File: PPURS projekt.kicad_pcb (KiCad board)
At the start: 2 copper layers, 80.5 x 53.5 mm, 26 parts, among them J3 Barrel_Jack, SW1 SW_Push_Dual, Y1 8Mhz

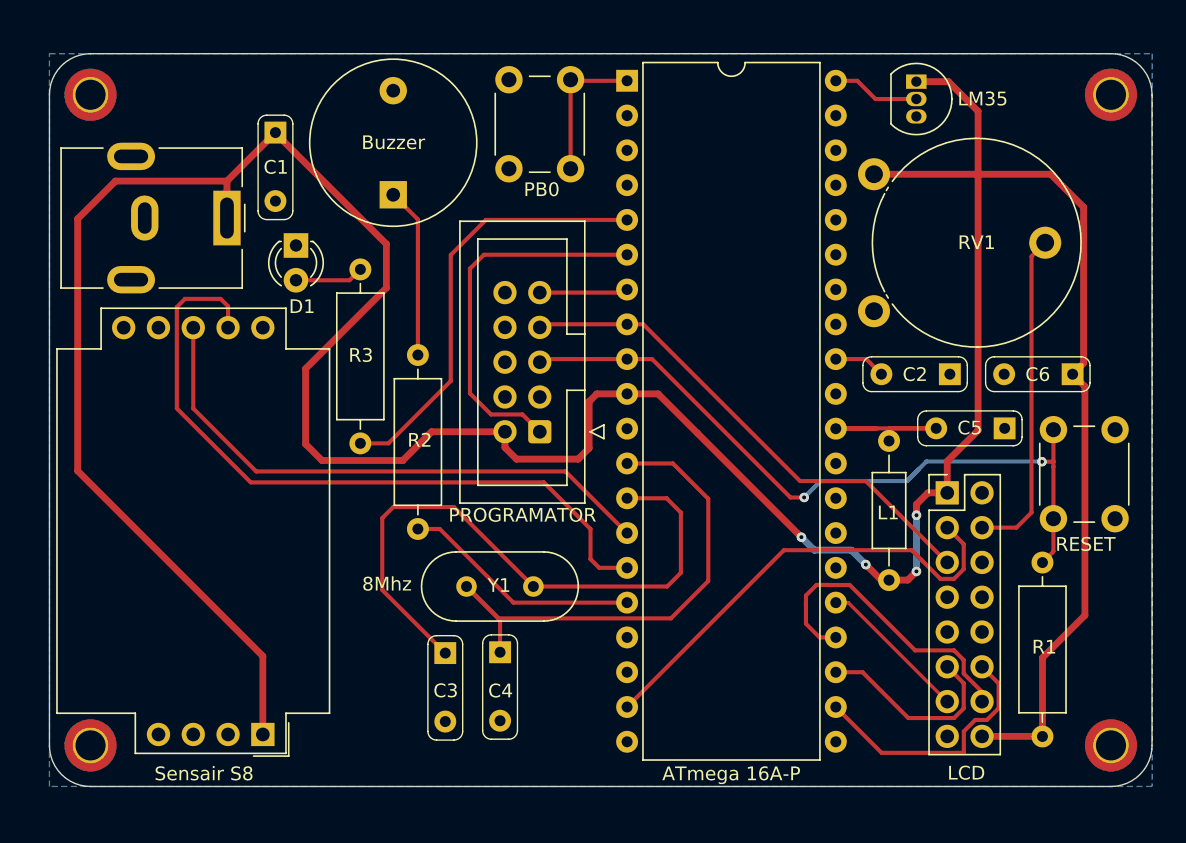
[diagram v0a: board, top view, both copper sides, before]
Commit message: Add files via upload
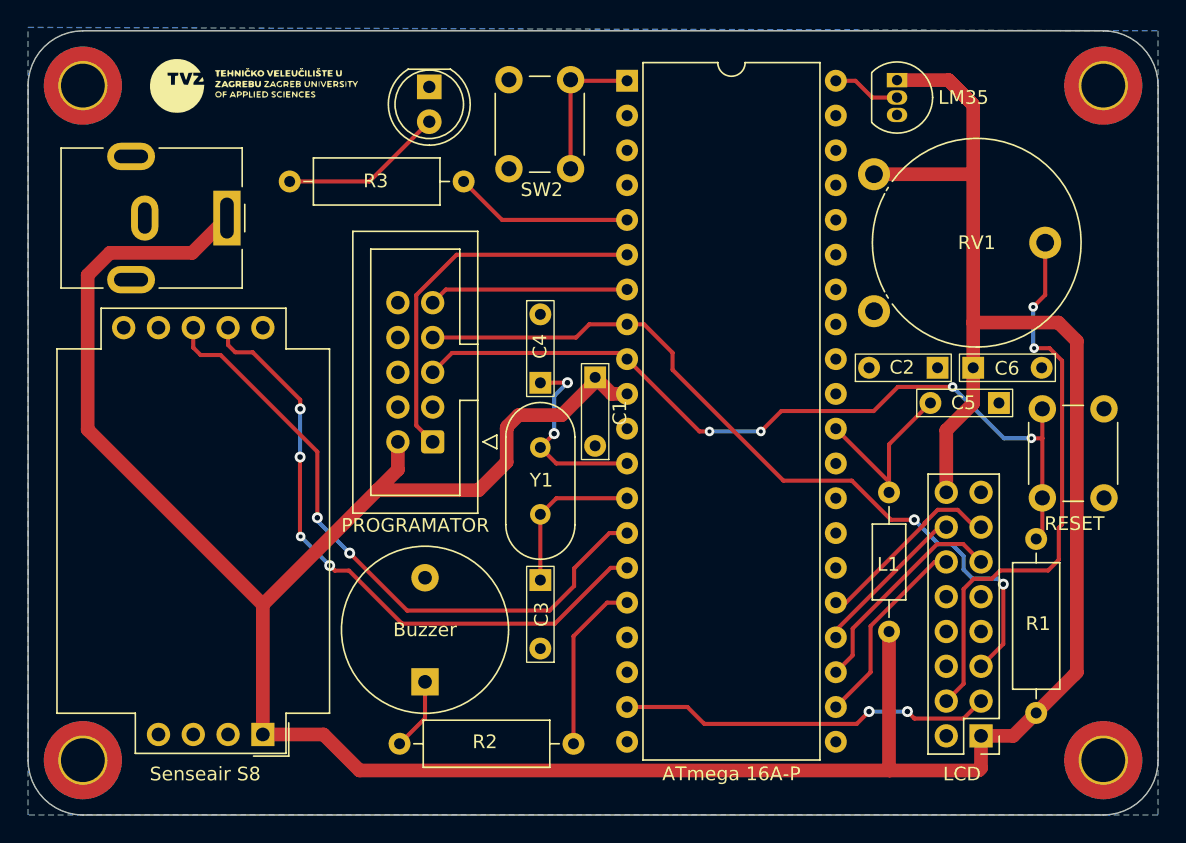
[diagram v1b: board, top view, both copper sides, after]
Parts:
- added G***: LOGO, Library:tvz logo, F.Cu at (123.0, 68.0)
- added G***: LOGO, Library:tvz logo, B.Cu at (118.0, 105.2)
- C1, C2, C3, C4, C5, C6: footprint Library:CP_Radial_Tantal_D5.0mm_P5.00mmjm -> Library:CP_Radial_Tantal_D5.0mm_P5.00mmJM
- D1: footprint LED_THT:LED_D3.0mm_FlatTop -> LED_THT:LED_D5.0mm_Clear
- H1, H2, H3, H4: footprint MountingHole:MountingHole_2.2mm_M2_DIN965_Pad_TopBottom -> MountingHole:MountingHole_3.2mm_M3_ISO7380_Pad_TopBottom
- J3: footprint Library:BarrelJack_CUI_PJ-063AH_Horizontaljm -> Library:BarrelJack_CUI_PJ-063AH_HorizontalJM
- Senseair S8: renamed from Sensair S8
- moved H4 75.1 mm to (110.5, 117.2)
- moved H2 75.1 mm to (110.5, 68.0)
- moved H3 73.9 mm to (185.0, 117.2)
- moved H1 73.9 mm to (185.0, 68.0)
- moved BZ1 35.6 mm to (135.5, 111.5)
- moved C1 29.4 mm to (147.9, 89.3)
- moved R2 28.4 mm to (133.6, 116.0), turned to 0 degrees
- moved C4 19.9 mm to (143.9, 89.7), turned to 90 degrees
- moved LCD 17.9 mm to (176.1, 115.5), turned to 180 degrees
- moved D1 15.1 mm to (135.8, 68.1)
- moved Y1 11.5 mm to (143.9, 94.4), turned to -90 degrees
- moved C3 8.75 mm to (143.9, 104.1)
- moved R3 8.24 mm to (125.6, 75.0), turned to 0 degrees
- moved PROGRAMATOR 7.85 mm to (136.0, 94.0)
- moved C6 7.28 mm to (175.5, 88.6), turned to 0 degrees
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- renumbered PB0 to SW2, LM35 to U3
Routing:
- net Net-(U1-XTAL1): track 45.5 -> 11.6 mm
- net Net-(U1-XTAL2): track 38.6 -> 14.4 mm, vias 0 -> 2
- net /PB7: track 37.0 -> 57.9 mm, vias 0 -> 2
- net Net-(U1-PB4): track 31.6 -> 13.1 mm
- net Net-(U4-VO): track 24.2 -> 41.7 mm, vias 0 -> 2
- net /PC2: track 22.6 -> 11.7 mm
- net +5V: track 251.9 -> 243.0 mm, vias 4 -> 0
- net /PB6: track 6.47 -> 14.6 mm
- net Net-(BZ1--): track 12.4 -> 5.29 mm
- net Net-(D1-A): track 5.03 -> 12.0 mm
- net /PD5: track 34.0 -> 27.5 mm, vias 0 -> 2
- net /RESET: track 54.2 -> 60.1 mm, vias 2 -> 4
- net /PD1 tx: track 52.2 -> 46.4 mm, vias 0 -> 4
- net /PD0 rx: track 41.3 -> 47.1 mm, vias 0 -> 2
- net Net-(U1-PD2): track 17.5 -> 12.8 mm
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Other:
- board size 80.5 x 53.5 mm -> 82.5 x 57.2 mm
- board text removed: "C3"
